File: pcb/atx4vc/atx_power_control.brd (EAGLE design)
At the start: 86 x 70 mm, 59 parts, among them IC2 REG1117, IC3 STM32F042F4, IC4 MY_7905DT, J1 ATX24RH, SW1 324_SW, SW2 324_SW, SW3 324_SW, SW4 324_SW, SW5 324_SW, SW7 324_SW, U1 USBC_16P, U2 USBC_16P

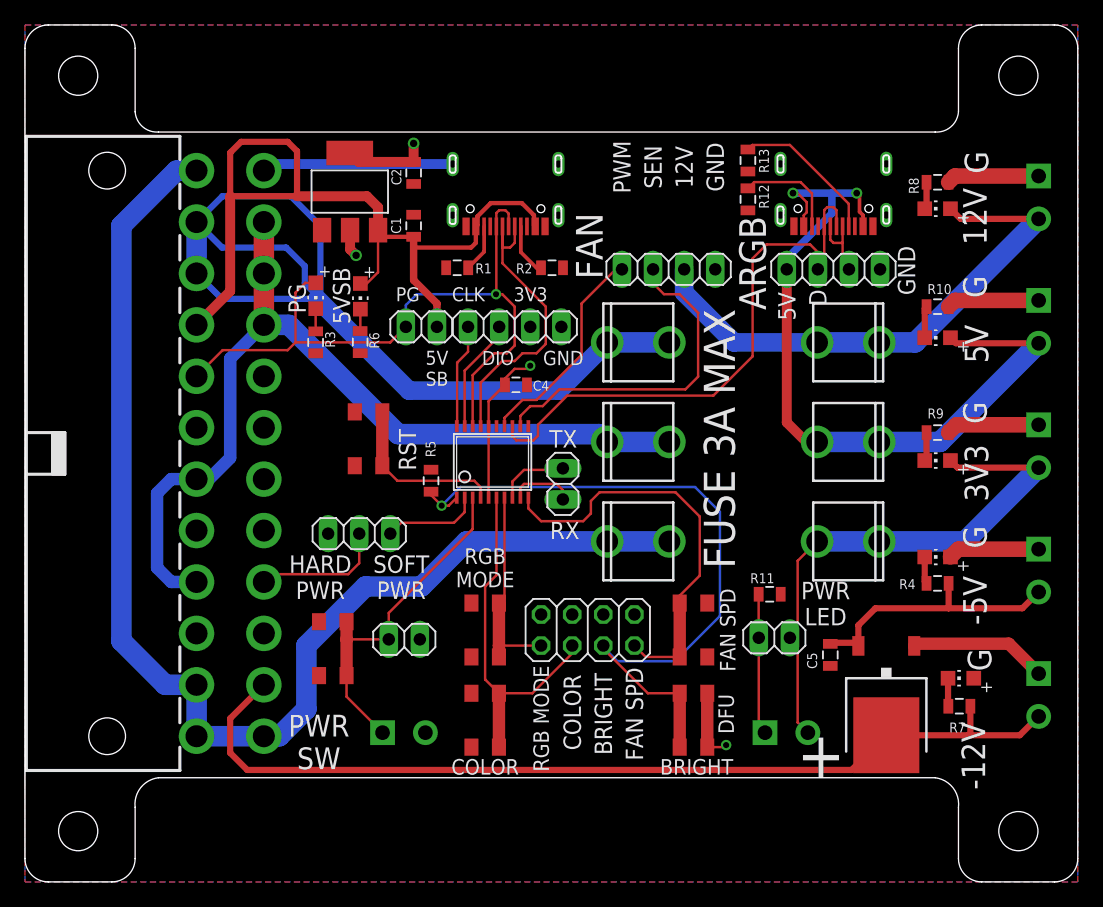
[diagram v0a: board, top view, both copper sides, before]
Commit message: updated pcb headers
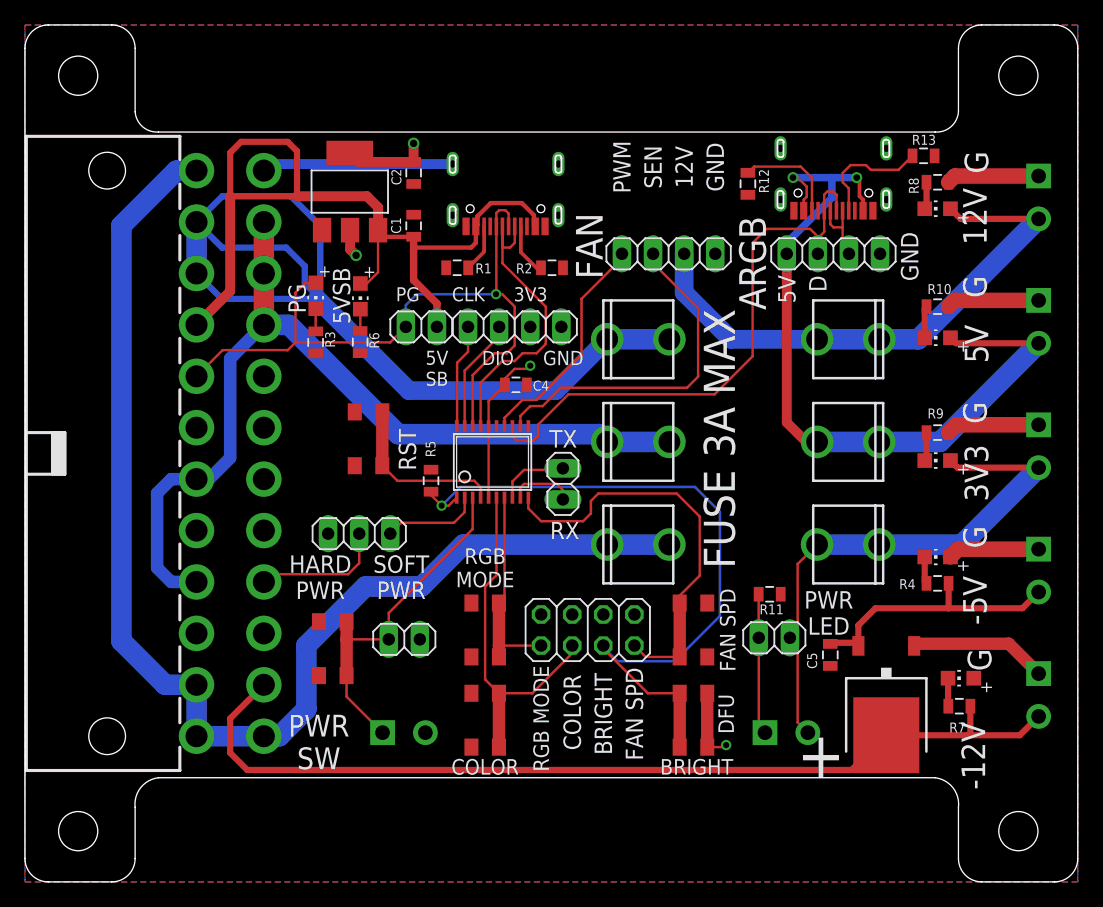
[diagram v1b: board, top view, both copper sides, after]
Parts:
- moved R13 14.4 mm to (73.4, 59.3), turned to 0 degrees
- moved JP2 1.27 mm to (52.6, 51.3)
- moved JP7 1.27 mm to (66.0, 51.3)
- moved R12 1.27 mm to (59.1, 57.0)
- moved U1 1.27 mm to (66.0, 58.7)
- moved F2 0.25 mm to (58.7, 44.3)
- moved F3 0.25 mm to (58.7, 27.6)
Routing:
- net N$34: track 12.2 -> 9.89 mm
- net N$35: track 47.0 -> 48.3 mm
- net N$15: track 63.8 -> 65.1 mm
- net N$16: track 44.3 -> 45.3 mm
- net N$7: track 17.8 -> 18.7 mm
- net N$6: track 27.7 -> 28.2 mm
